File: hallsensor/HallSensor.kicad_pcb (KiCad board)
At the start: 2 copper layers, 6.3 x 20.3 mm, 5 parts

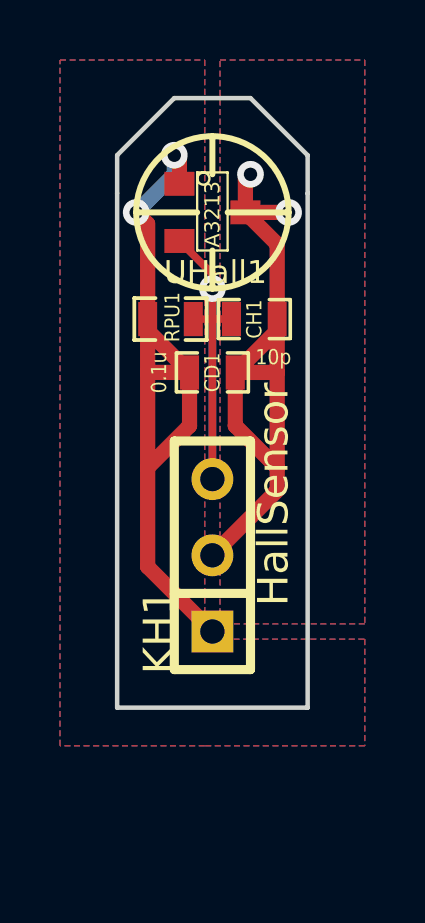
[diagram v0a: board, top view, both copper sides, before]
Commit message: Misc rework.
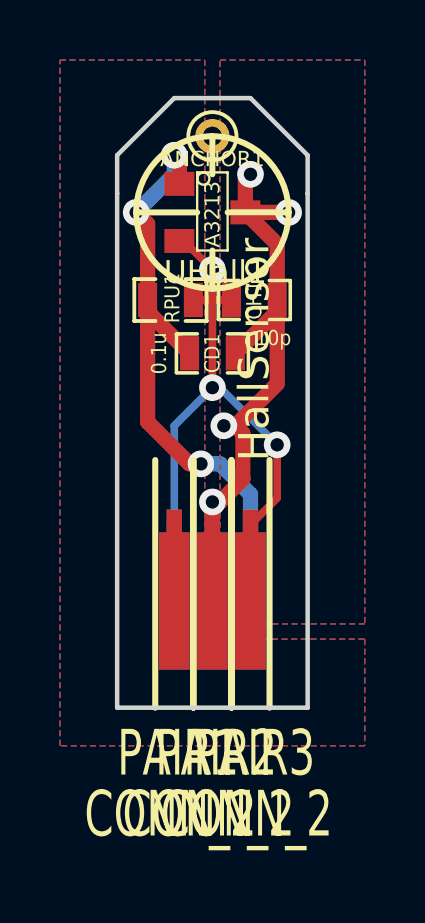
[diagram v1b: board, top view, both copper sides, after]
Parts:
- removed KH1: CONN_3, SIL-3
- added ANCHOR1: CONN_1, PINTST, F.Cu at (25.4, 22.9)
- added PAIR1: CONN_2, EDGE_2, F.Cu at (24.1, 38.1)
- added PAIR2: CONN_2, EDGE_2, F.Cu at (25.4, 38.1)
- added PAIR3: CONN_2, EDGE_2, F.Cu at (26.7, 38.1)
- moved CD1 0.64 mm to (25.4, 30.1)
- moved CH1 0.63 mm to (26.8, 28.3)
- moved RPU1 0.63 mm to (24.0, 28.3)
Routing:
- net /hall1: track 16.0 -> 23.1 mm, vias 1 -> 3
- net VCC: track 26.0 -> 23.7 mm, vias 2 -> 3
- net VSS: track 23.1 -> 22.8 mm, vias 2 -> 4
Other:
- net class Default: clearance 0.254 -> 0.2032
- net class PWR_Nets: clearance 0.254 -> 0.2032
- rule trace_clearance: 0.254 -> 0.2032
